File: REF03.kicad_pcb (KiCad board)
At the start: 2 copper layers, 45 x 45 mm, 20 parts, among them SW1 SW_SPST, U1 SN74LVC2G14DBV, U2 REF03GP

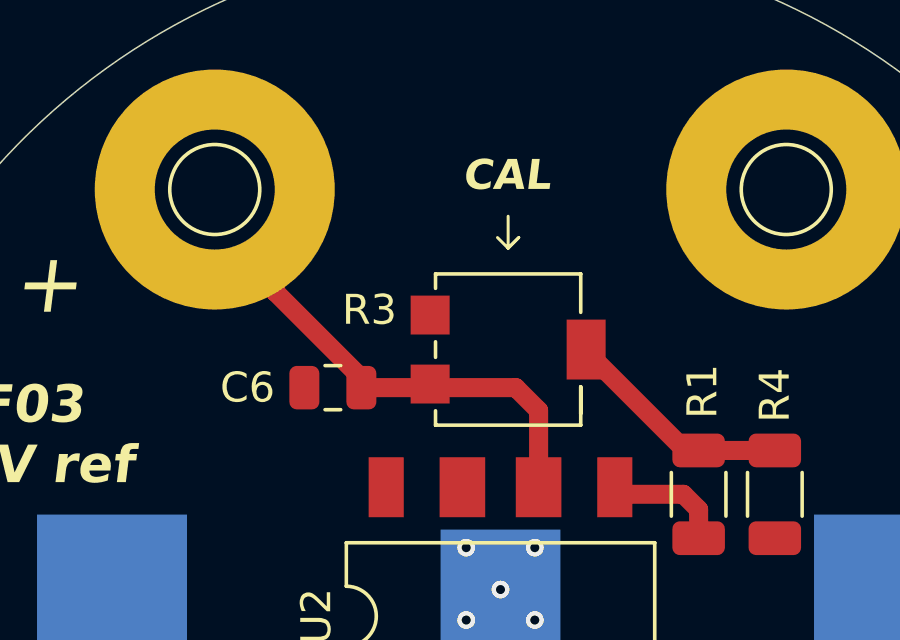
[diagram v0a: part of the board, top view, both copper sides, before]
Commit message: Updated README
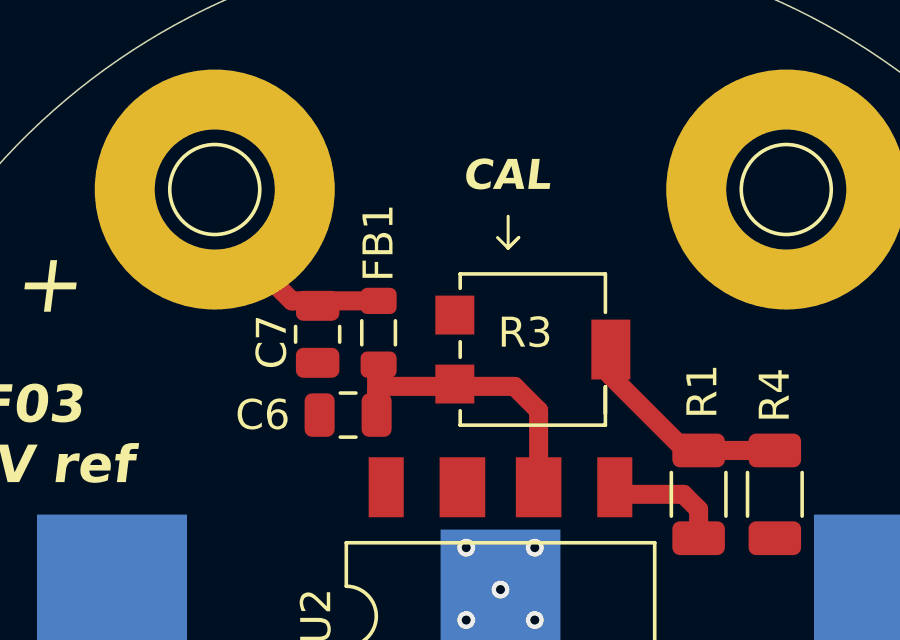
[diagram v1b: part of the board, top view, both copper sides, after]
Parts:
- added C7: 10u, Capacitor_SMD:C_0805_2012Metric, F.Cu at (-6.10, -9.40)
- added FB1: FerriteBead, Inductor_SMD:L_0805_2012Metric, F.Cu at (-4.06, -9.45)
- moved C6 1.05 mm to (-5.08, -6.71)
- moved R3 0.82 mm to (1.08, -8.89)
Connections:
- TP1 pad 1: Net-(U2-VOUT) -> Net-(C7-Pad2)
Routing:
- net Net-(C7-Pad2): track 0.00 -> 7.67 mm
- net Net-(U2-VOUT): track 15.6 -> 11.1 mm
